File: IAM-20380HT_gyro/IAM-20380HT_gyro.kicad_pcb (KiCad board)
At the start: 2 copper layers, 21 x 24.9 mm, 7 parts, among them U1 IAM-20380

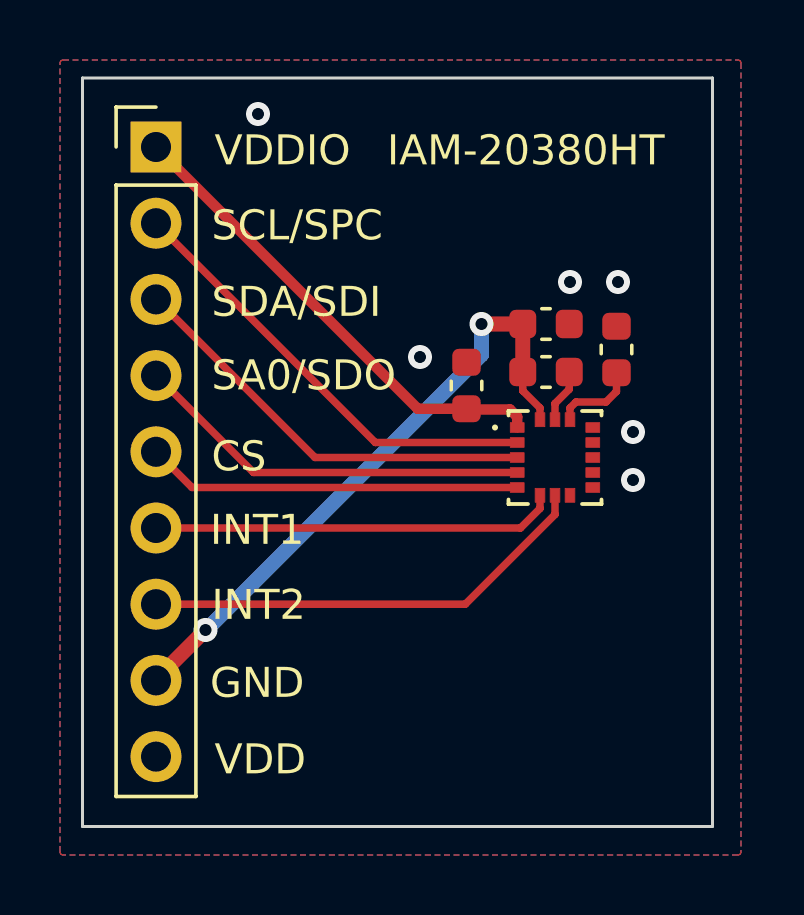
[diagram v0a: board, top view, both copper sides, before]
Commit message: created gerber stuff
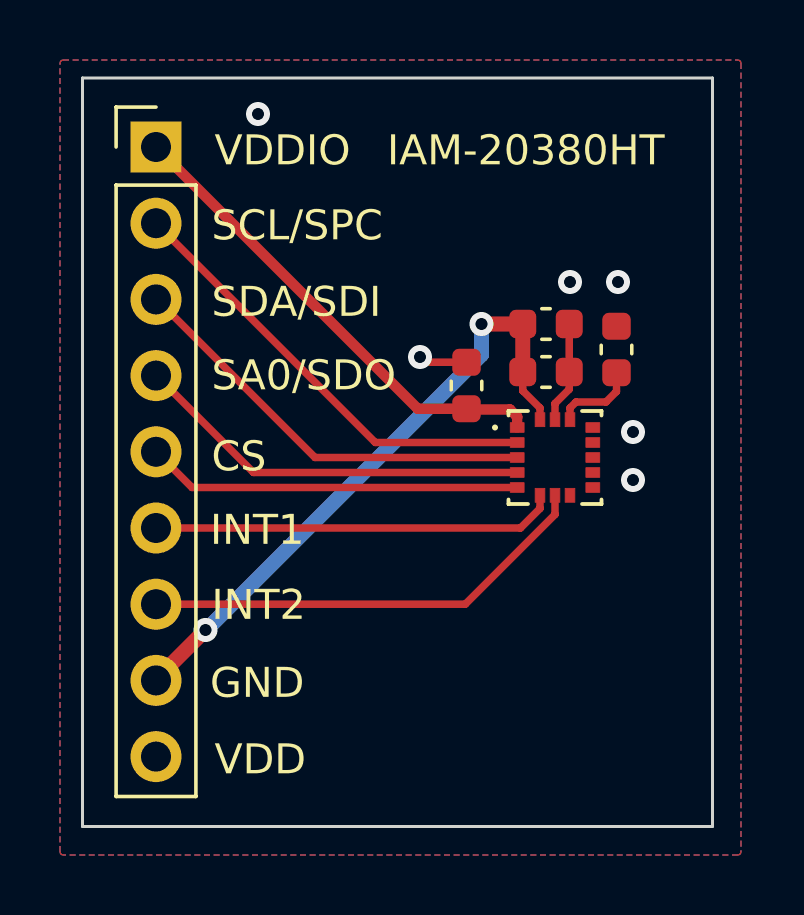
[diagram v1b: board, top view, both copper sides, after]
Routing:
- net GNDPWR: track 1.81 -> 5.01 mm
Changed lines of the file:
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@@
       (outputformat 1)
       (mirror false)
-      (drillshape 1)
+      (drillshape 0)
       (scaleselection 1)
       (outputdirectory "")
@@
   (segment (start 148.65 98.85) (end 148.65 98.225) (width 0.25) (layer "F.Cu") (net 1))
   (segment (start 147.1 99.79) (end 147.1 99.4) (width 0.25) (layer "F.Cu") (net 1))
-  (segment (start 133.3 111) (end 133.3 111.02) (width 0.5) (layer "F.Cu") (net 2))
+  (segment (start 143.65 97.875) (end 142.275 97.875) (width 0.25) (layer "F.Cu") (net 2))
   (segment (start 146.6 99.79) (end 146.6 99.25) (width 0.25) (layer "F.Cu") (net 2))
   (segment (start 146.6 99.25) (end 147.075 98.775) (width 0.25) (layer "F.Cu") (net 2))
+  (segment (start 142.275 97.875) (end 142.1 97.7) (width 0.25) (layer "F.Cu") (net 2))
+  (segment (start 147.075 98.2) (end 147.075 96.6) (width 0.25) (layer "F.Cu") (net 2))
   (segment (start 147.075 98.775) (end 147.075 98.2) (width 0.25) (layer "F.Cu") (net 2))
   (via (at 149.2 101.8) (size 0.8) (drill 0.4) (layers "F.Cu" "B.Cu") (free) (net 2))
